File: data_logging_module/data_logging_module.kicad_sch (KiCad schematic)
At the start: 4 parts

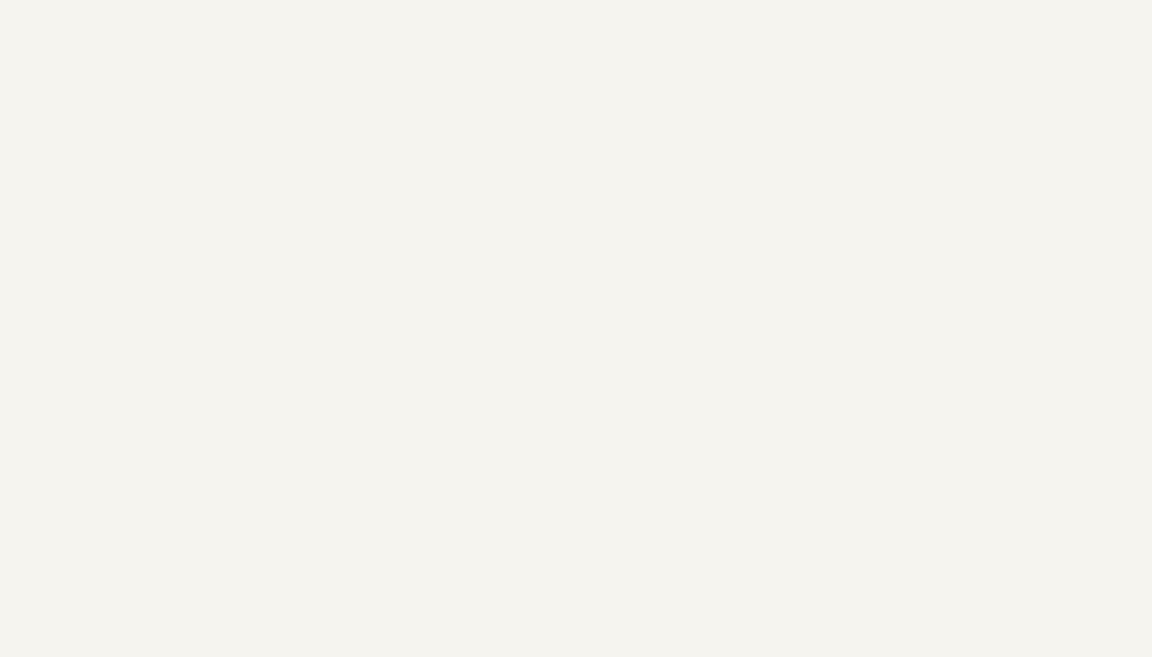
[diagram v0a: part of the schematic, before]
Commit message: Initial scheme
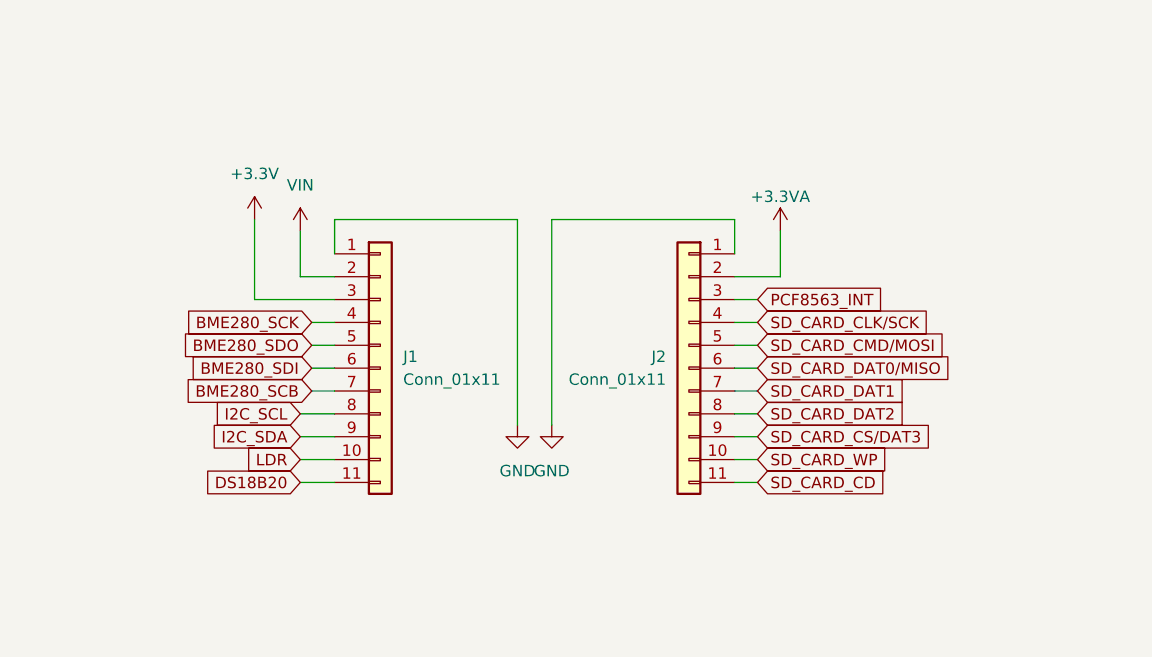
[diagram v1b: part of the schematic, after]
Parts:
- added J1, J2: Conn_01x11, Connector_PinHeader_2.54mm:PinHeader_1x11_P2.54mm_Vertical, symbol Connector_Generic:Conn_01x11
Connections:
- new net +3.3V: J1.3 (Pin_3)
- new net +3.3VA: J2.2 (Pin_2)
- new net BME280_SCB: J1.7 (Pin_7)
- new net BME280_SCK: J1.4 (Pin_4)
- new net BME280_SDI: J1.6 (Pin_6)
- new net BME280_SDO: J1.5 (Pin_5)
- new net DS18B20: J1.11 (Pin_11)
- new net GND: J1.1 (Pin_1), J2.1 (Pin_1)
- new net I2C_SCL: J1.8 (Pin_8)
- new net I2C_SDA: J1.9 (Pin_9)
- new net LDR: J1.10 (Pin_10)
- new net PCF8563_INT: J2.3 (Pin_3)
- new net SD_CARD_CD: J2.11 (Pin_11)
- new net SD_CARD_CLK/SCK: J2.4 (Pin_4)
- new net SD_CARD_CMD/MOSI: J2.5 (Pin_5)
- new net SD_CARD_CS/DAT3: J2.9 (Pin_9)
- new net SD_CARD_DAT0/MISO: J2.6 (Pin_6)
- new net SD_CARD_DAT1: J2.7 (Pin_7)
- new net SD_CARD_DAT2: J2.8 (Pin_8)
- new net SD_CARD_WP: J2.10 (Pin_10)
- new net VIN: J1.2 (Pin_2)
